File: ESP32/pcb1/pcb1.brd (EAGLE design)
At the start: 100 x 80 mm, 0 parts

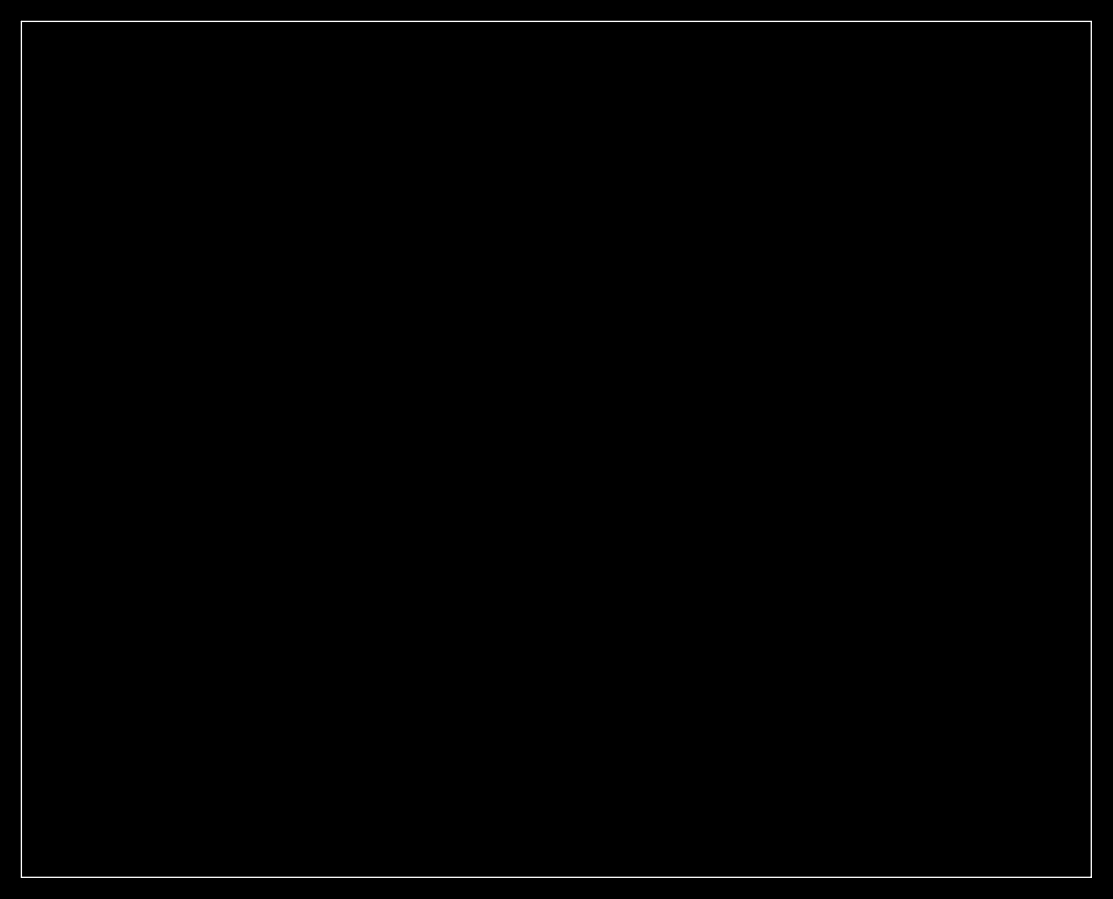
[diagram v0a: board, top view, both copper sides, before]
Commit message: UPD: ESP32/pcb1
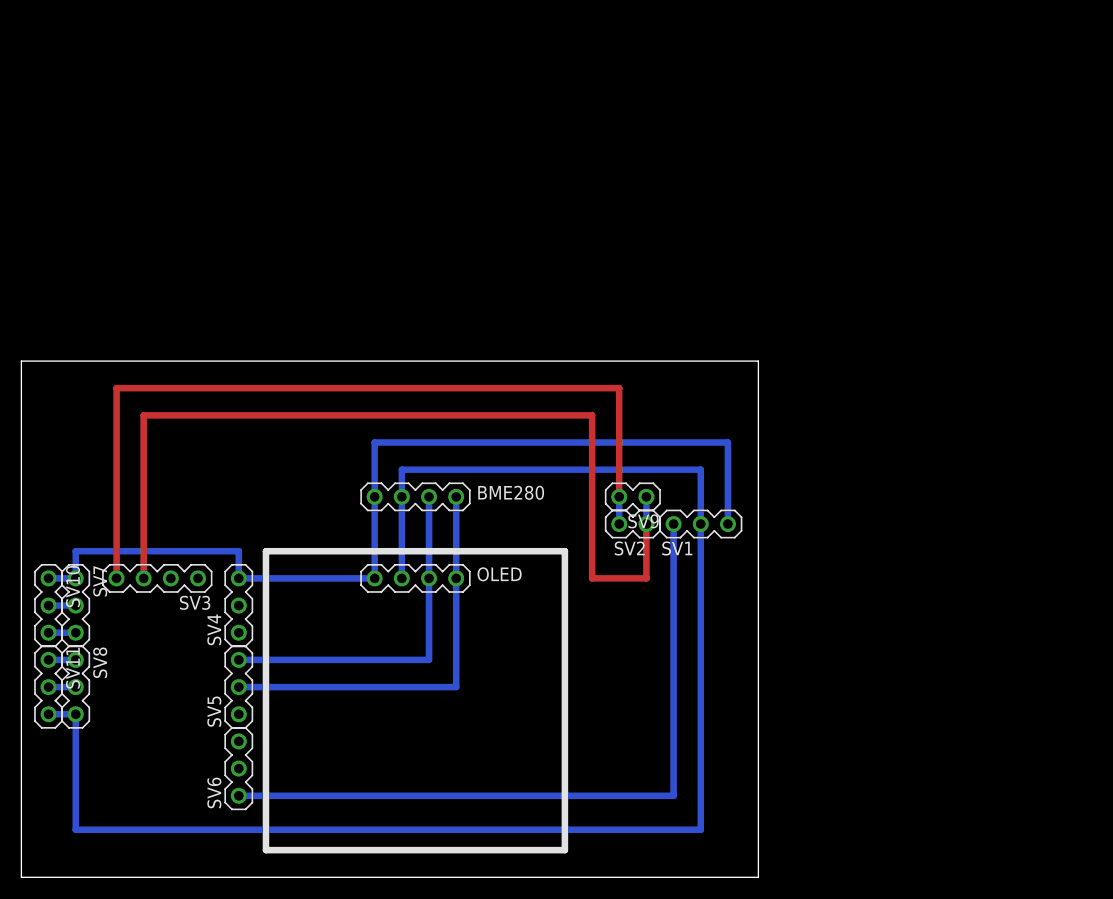
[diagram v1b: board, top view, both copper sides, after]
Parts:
- added BME280, OLED, SV3: (no value), ytani1:PINHEAD-MA04-1
- added SV1, SV10, SV11, SV4, SV5, SV6, SV7, SV8: (no value), ytani1:PINHEAD-MA03-1
- added SV2, SV9: (no value), ytani1:PINHEAD-MA02-1
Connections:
- new net +3V3: BME280.2, OLED.3, SV1.2, SV11.3, SV8.3
- new net GND: BME280.1, OLED.4, SV1.1, SV10.1, SV4.3, SV7.1
- new net N$1: SV1.3, SV6.1
- new net N$2: BME280.3, OLED.2, SV5.3
- new net N$3: BME280.4, OLED.1, SV5.2
- new net N$4: SV10.2, SV7.2
- new net N$5: SV2.2, SV3.4, SV9.2
- new net N$6: SV2.1, SV3.3, SV9.1
- new net N$7: SV10.3, SV7.3
- new net N$8: SV11.1, SV8.1
- new net N$9: SV11.2, SV8.2
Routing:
- net +3V3: track 0.00 -> 143.5 mm
- net GND: track 0.00 -> 88.9 mm
- net N$6: track 0.00 -> 85.1 mm
- net N$5: track 0.00 -> 77.5 mm
- net N$1: track 0.00 -> 66.0 mm
- net N$3: track 0.00 -> 38.1 mm
- net N$2: track 0.00 -> 33.0 mm
- net N$9: track 0.00 -> 2.54 mm
- net N$8: track 0.00 -> 2.54 mm
- net N$7: track 0.00 -> 2.54 mm
- net N$4: track 0.00 -> 2.54 mm
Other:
- board size 100 x 80 mm -> 68.9 x 48.2 mm
